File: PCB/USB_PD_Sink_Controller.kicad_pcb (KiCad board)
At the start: 2 copper layers, 43.5 x 30.8 mm, 27 parts, among them J1 USB_C_Receptacle_PowerOnly_6P, J2 JST_01x02_Socket, U1 STUSB4500QTR, U2 STL6P3LLH6, U3 STL6P3LLH6

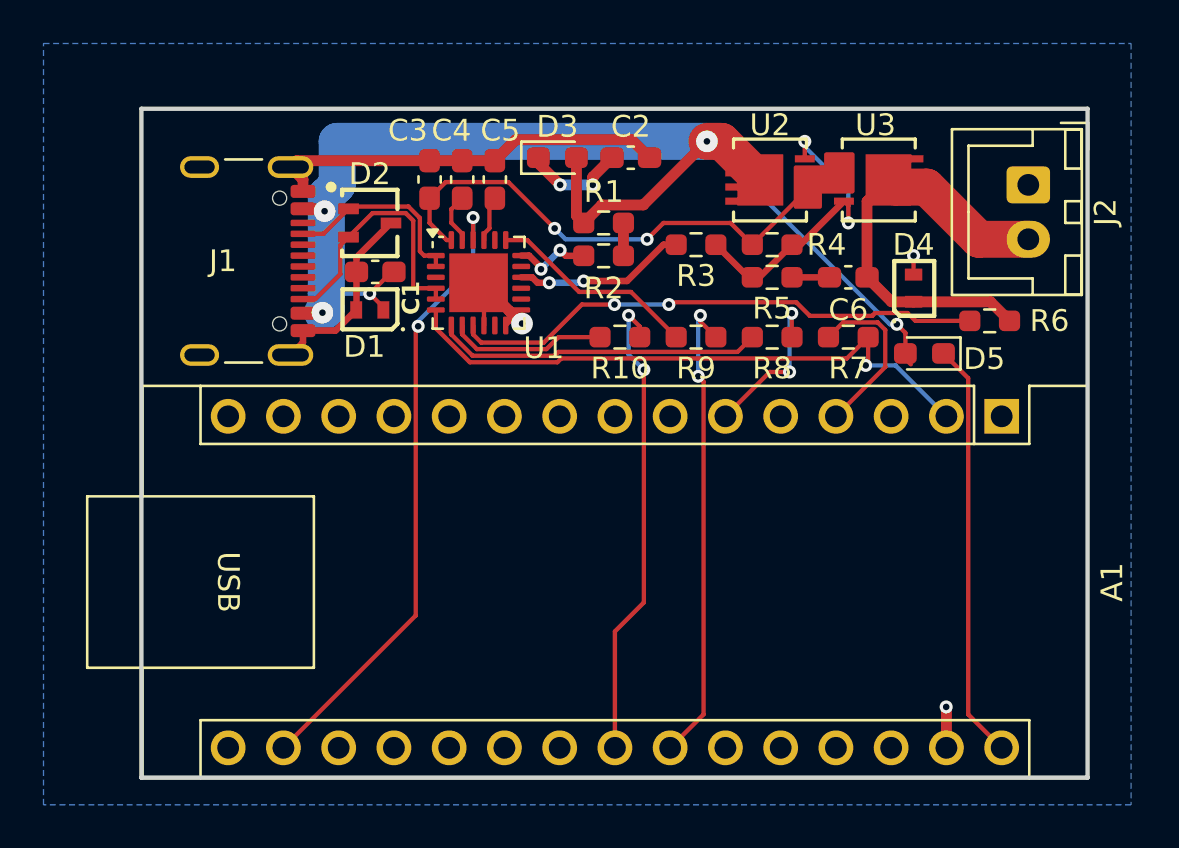
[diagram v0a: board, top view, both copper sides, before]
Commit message: Updated PCB
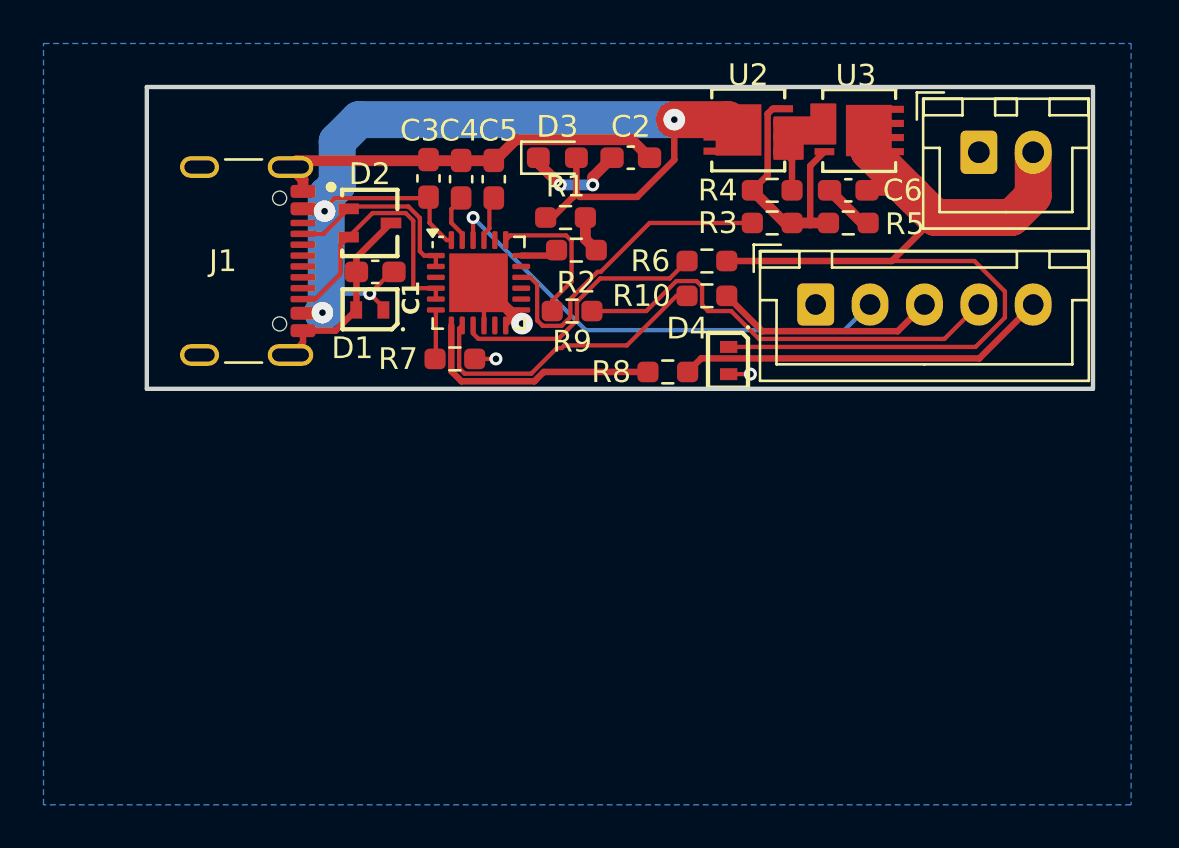
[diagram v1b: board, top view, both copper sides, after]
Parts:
- removed A1: Arduino_Nano_ESP32, Module:Arduino_Nano
- removed D5: D, Diode_SMD:D_0603_1608Metric_Pad1.05x0.95mm_HandSolder
- added J3: JST_01x05_Socket, Connector_JST:JST_XH_B5B-XH-A_1x05_P2.50mm_Vertical, F.Cu at (345.5, 122.0)
- moved R7 18.1 mm to (328.9, 124.5)
- moved R6 13.3 mm to (340.5, 120.0)
- moved D4 9.13 mm to (341.5, 124.6), turned to -90 degrees
- moved R9 5.82 mm to (334.3, 122.3), turned to 0 degrees
- moved R8 5.06 mm to (338.7, 125.1)
- moved R10 4.43 mm to (340.5, 121.6), turned to 0 degrees
- moved R5 4.30 mm to (347.0, 118.2)
- moved C6 4.00 mm to (347.0, 116.8)
- moved R3 3.64 mm to (343.5, 118.2)
- moved J2 2.72 mm to (353.0, 115.0), turned to 0 degrees
- moved U2 2.51 mm to (342.4, 114.0)
- moved R4 2.50 mm to (343.5, 116.8), turned to 0 degrees
- moved U3 2.45 mm to (347.5, 114.0)
- moved R1 1.77 mm to (334.0, 118.0)
- moved R2 1.28 mm to (334.5, 119.5)
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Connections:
- C1 pad 1: /Vbus -> /VDD
- C3 pad 1: GND -> /VDD
- C3 pad 2: /VDD -> GND
- C4 pad 1: GND -> Net-(U1-VREG_2V7)
- C4 pad 2: Net-(U1-VREG_2V7) -> GND
- C5 pad 1: GND -> Net-(U1-VREG_1V2)
- C5 pad 2: Net-(U1-VREG_1V2) -> GND
- D1 pad 1: /Vbus -> /VDD
- D3 pad 2: /Vbus -> /VDD
- J1 pad A9: /Vbus -> /VDD
- J1 pad B9: /Vbus -> /VDD
- R1 pad 1: /Vbus -> /VDD
- R10 pad 1: Net-(A1-SDA/A4) -> Net-(U1-SDA)
- R4 pad 2: /VDD -> Net-(U2-S)
- R7 pad 1: /RESET -> GND
- R7 pad 2: GND -> /RESET
- R8 pad 1: Net-(A1-D3) -> /ALERT
- R8 pad 2: /ALERT -> Net-(U1-SCL)
- R9 pad 1: Net-(A1-SCL/A5) -> Net-(U1-ALERT)
- U1 pad 19: /SCL -> Net-(U1-ALERT)
- U1 pad 22: /VSYS -> /3V3
- U1 pad 7: /ALERT -> Net-(U1-SCL)
- U1 pad 8: /SDA -> Net-(U1-SDA)
- U2 pad 2: /VDD -> Net-(U2-S)
- U2 pad 3: /Vbus -> /VDD
- U3 pad 2: /VDD -> Net-(U2-S)
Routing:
- net /Vbus: track 59.1 -> 0.00 mm, vias 5 -> 0
- net /VDD: track 22.7 -> 52.0 mm, vias 2 -> 4
- net /VSYS: track 29.0 -> 0.00 mm, vias 2 -> 0
- net /RESET: track 27.9 -> 2.48 mm, vias 1 -> 0
- net Net-(D4-K): track 19.8 -> 44.7 mm
- net /3V3: track 0.00 -> 22.2 mm, vias 0 -> 1
- net Net-(A1-SCL/A5): track 22.0 -> 0.00 mm, vias 2 -> 0
- net Net-(A1-SDA/A4): track 21.9 -> 0.00 mm, vias 2 -> 0
- net Net-(A1-VIN): track 19.2 -> 0.00 mm
- net Net-(U1-SDA): track 0.00 -> 14.1 mm
- net /DISCH: track 24.7 -> 12.3 mm, vias 2 -> 0
- net Net-(U1-SCL): track 0.00 -> 11.5 mm
- net /SCL: track 9.69 -> 20.6 mm
- net GND: track 44.9 -> 36.2 mm
- net Net-(A1-D3): track 7.64 -> 0.00 mm, vias 2 -> 0
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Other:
- board size 43.5 x 30.8 mm -> 43.5 x 13.9 mm
- board text added: "3V3"
- board text added: "ALT"
- board text added: "GND"
- board text added: "SCL"
- board text added: "SDA"
- board text added: "VBUS"
